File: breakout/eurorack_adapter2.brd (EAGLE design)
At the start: 22.8 x 22.9 mm, 12 parts, among them SW1 HEADER/MALE/01, SW2 HEADER/MALE/01, SW3 HEADER/MALE/01, SW4 HEADER/MALE/01

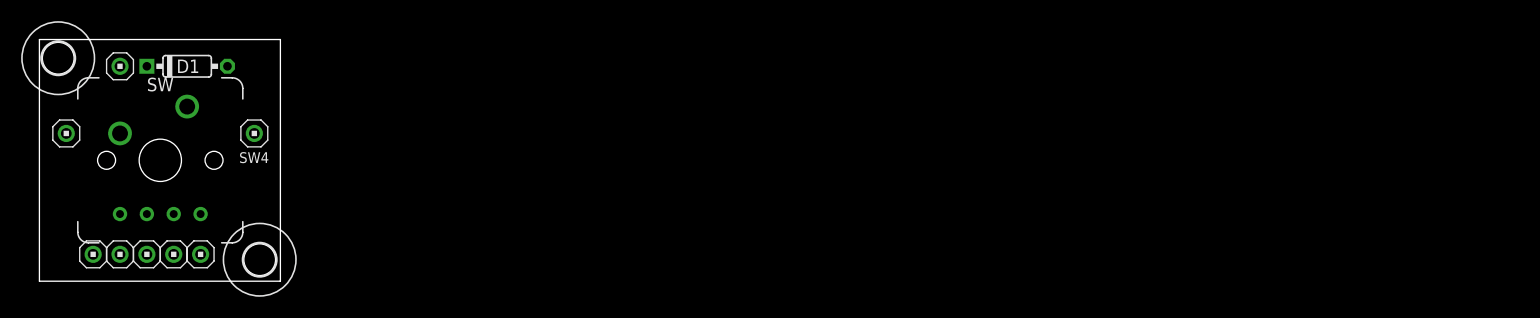
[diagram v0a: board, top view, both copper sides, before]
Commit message: Changes
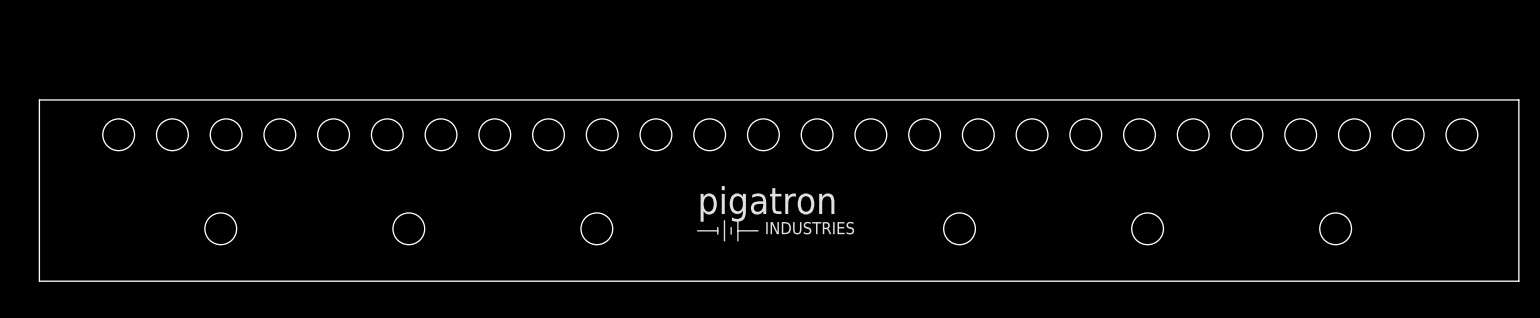
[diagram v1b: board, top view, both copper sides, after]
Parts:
- removed B, C, G, R, SW1, SW2, SW3, SW4: HEADER/MALE/01, connectors:HEADER/MALE/01
- removed D1: (no value), transistors:DO35-7
- removed SW: SWITCH_CHERRY_MX_RGBSWITCH_CHERRY_MX_RGB, controls:SWITCH_CHERRY_MX_RGB
- removed U$2: (no value), mechanical:STANDOFF/3.0
- U$1: device mechanical:STANDOFF/3.0 -> mechanical:PIGATRON-LOGO
- moved U$1 50.5 mm to (71.1, 6.35)
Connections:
- removed net N$1: SW.1, SW1.1, SW4.1
- removed net N$2: D1.A, SW.2
- removed net N$3: B.1, SW.B
- removed net N$4: G.1, SW.G
- removed net N$5: R.1, SW.R
- removed net N$6: C.1, SW.CA
- removed net N$7: D1.C, SW2.1, SW3.1
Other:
- board size 22.8 x 22.9 mm -> 139.9 x 17.1 mm
